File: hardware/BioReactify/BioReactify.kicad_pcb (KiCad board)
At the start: 4 copper layers, 110 x 110 mm, 131 parts, among them IC4 MJ5688-B111-HR1-C, J1 Conn_01x02, J10 Conn_01x06_Pin, J11 Conn_01x04_Pin, J12 Conn_01x04_Pin, J13 Conn_01x04_Pin, J14 Conn_01x04_Pin, J16 KF25C-7.62-2P, J17 Conn_01x02, J18 Conn_01x02, J19 Conn_01x02, J2 Conn_01x02, J20 Conn_01x02, J21 Conn_01x02, J22 Conn_01x02, J23 Conn_01x02, J24 Conn_01x03, J3 Conn_01x02, J4 Conn_01x02, J5 Conn_01x02, J6 Conn_01x03, J7 Conn_01x03, J8 Conn_01x02, J9 Conn_01x06_Pin, Q1 IRLZ44N, Q2 IRLZ44N, Q3 IRLZ44N, Q4 IRLZ44N, Q5 IRLZ44N, U1 LD1117S33TR_SOT223, U10 4N25, U11 4N25, U12 LD1117S50TR_SOT223, U13 MAX3490xSA, U14 TLV9001IDCK, U15 TLV9001IDCK, U16 TLV9001IDCK, U17 LD1117S33TR_SOT223, U18 MCP3208, U2 TLV9001IDCK, U3 TCA9544A, U4 TLV9001IDCK, U5 ESP32-DEVKIT-V1, U6 ACS712xLCBTR-030B3, U7 4N25, U8 4N25, U9 4N25

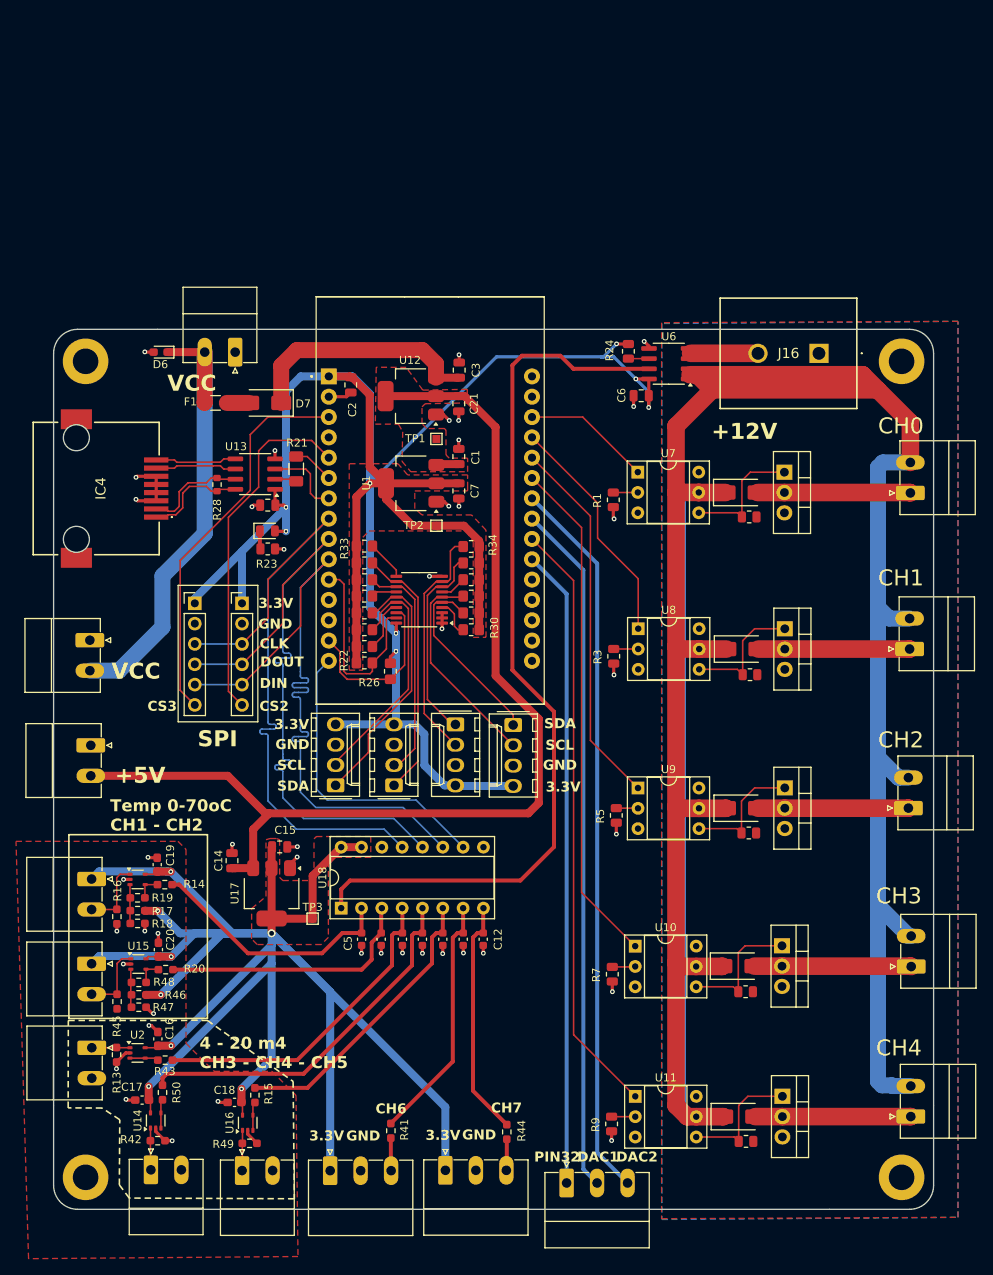
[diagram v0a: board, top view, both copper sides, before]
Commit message: Hardware updated
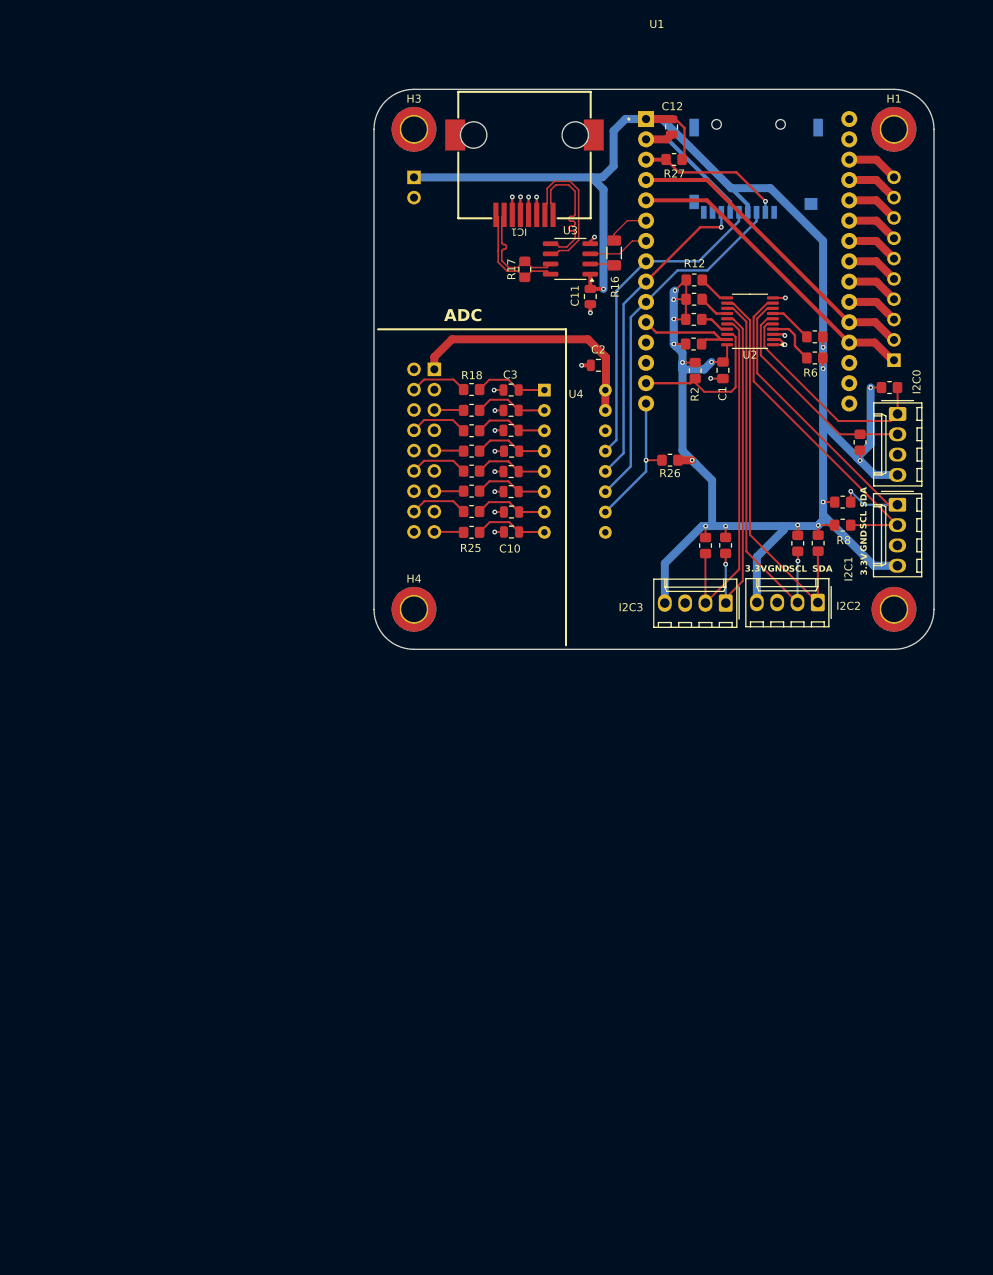
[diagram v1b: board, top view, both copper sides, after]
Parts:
- removed C13: 0.047uf, Capacitor_SMD:C_0603_1608Metric
- removed C14: 100nF, Capacitor_SMD:C_0805_2012Metric
- removed C15, C21: 10uF, Capacitor_SMD:C_0805_2012Metric
- removed C16, C17, C18, C19, C20: 0.1uF, Capacitor_SMD:C_0603_1608Metric_Pad1.08x0.95mm_HandSolder
- removed D1, D2, D3, D4, D5: 50V 5A, Diode_SMD:D_SMA
- removed D6: VS12VBA1HS, Diode_SMD:D_0603_1608Metric_Pad1.05x0.95mm_HandSolder
- removed D7: B340A-13-F, Diode_SMD:D_SMA
- removed D9: LED, LED_SMD:LED_0805_2012Metric
- removed F1: 13.2V 3A, Fuse:Fuse_1206_3216Metric
- removed IC4: MJ5688-B111-HR1-C, SamacSys_Parts:MJ5688B111HR1C
- removed J10, J9: Conn_01x06_Pin, Connector_PinHeader_2.54mm:PinHeader_1x06_P2.54mm_Vertical
- removed J11, J12, J13, J14: Conn_01x04_Pin, Connector_Molex:Molex_KK-254_AE-6410-04A_1x04_P2.54mm_Vertical
- removed J16: KF25C-7.62-2P, SamacSys_Parts:KF25C7622P
- removed J17, J18, J19, J20, J21, J22, J23, J5, J8: Conn_01x02, Connector_Phoenix_MC:PhoenixContact_MC_1,5_2-G-3.81_1x02_P3.81mm_Horizontal
- removed J24, J6, J7: Conn_01x03, Connector_Phoenix_MC:PhoenixContact_MC_1,5_3-G-3.81_1x03_P3.81mm_Horizontal
- removed Q1, Q2, Q3, Q4, Q5: IRLZ44N, Package_TO_SOT_THT:TO-220-3_Vertical
- removed R28: 120, Resistor_SMD:R_0603_1608Metric
- removed R29, R30, R31, R32, R33, R34, R35, R36, R37, R38, R39, R40: 10K, Resistor_SMD:R_0805_2012Metric_Pad1.20x1.40mm_HandSolder
- removed R41, R43, R44, R50: 1K, Resistor_SMD:R_0603_1608Metric_Pad0.98x0.95mm_HandSolder
- removed R42, R49: 150, Resistor_SMD:R_0603_1608Metric_Pad0.98x0.95mm_HandSolder
- removed R45: 7.8K, Resistor_SMD:R_0603_1608Metric_Pad0.98x0.95mm_HandSolder
- removed R46, R47: 4.1K, Resistor_SMD:R_0603_1608Metric_Pad0.98x0.95mm_HandSolder
- removed R48: 1.5K, Resistor_SMD:R_0603_1608Metric_Pad0.98x0.95mm_HandSolder
- removed TP1, TP2, TP3: TestPoint, TestPoint:TestPoint_Pad_1.0x1.0mm
- removed U10, U11, U7, U8, U9: 4N25, Package_DIP:DIP-6_W7.62mm_Socket
- removed U12: LD1117S50TR_SOT223, Package_TO_SOT_SMD:SOT-223-3_TabPin2
- removed U13: MAX3490xSA, Package_SO:SOIC-8_3.9x4.9mm_P1.27mm
- removed U14, U15, U16: TLV9001IDCK, Package_TO_SOT_SMD:SOT-353_SC-70-5
- removed U17: LD1117S33TR_SOT223, Package_TO_SOT_SMD:SOT-223-3_TabPin2
- removed U18: MCP3208, Package_DIP:DIP-16_W7.62mm_Socket
- removed U5: ESP32-DEVKIT-V1, other:MODULE_ESP32_DEVKIT_V1
- removed U6: ACS712xLCBTR-030B3, Package_SO:SOIC-8_3.9x4.9mm_P1.27mm
- added I2C0: Conn_01x04_Pin, Connector_Molex:Molex_KK-254_AE-6410-04A_1x04_P2.54mm_Vertical, F.Cu at (205.4, 60.6)
- added I2C1: Conn_01x04_Pin, Connector_Molex:Molex_KK-254_AE-6410-04A_1x04_P2.54mm_Vertical, F.Cu at (205.4, 71.9)
- added I2C2: Conn_01x04_Pin, Connector_Molex:Molex_KK-254_AE-6410-04A_1x04_P2.54mm_Vertical, F.Cu at (195.5, 84.2)
- added I2C3: Conn_01x04_Pin, Connector_Molex:Molex_KK-254_AE-6410-04A_1x04_P2.54mm_Vertical, F.Cu at (184.0, 84.2)
- added IC1: MJ5688-B111-HR1-C, custom:RJ45-TH_MJ5688-B111-HR1-C, F.Cu at (158.8, 30.7)
- added R11: 10K, Resistor_SMD:R_0805_2012Metric_Pad1.20x1.40mm_HandSolder, F.Cu at (193.0, 76.8)
- added R12: 10K, Resistor_SMD:R_0805_2012Metric_Pad1.20x1.40mm_HandSolder, F.Cu at (180.0, 43.8)
- added R25: 100, Resistor_SMD:R_0805_2012Metric_Pad1.20x1.40mm_HandSolder, F.Cu at (152.2, 75.4)
- C1: value 100nF -> 10uF; footprint Capacitor_SMD:C_0805_2012Metric -> Capacitor_SMD:C_0805_2012Metric_Pad1.18x1.45mm_HandSolder
- C10, C5, C8, C9: value 0.047uf -> 0.022uF; footprint Capacitor_SMD:C_0603_1608Metric -> Capacitor_SMD:C_0805_2012Metric
- C11, C12: value 0.047uf -> 10uF; footprint Capacitor_SMD:C_0603_1608Metric -> Capacitor_SMD:C_0805_2012Metric
- C3: value 100nF -> 0.022uF
- C4, C6, C7: value 10uF -> 0.022uF
- H1, H2, H3, H4: footprint MountingHole:MountingHole_3.2mm_M3_ISO7380_Pad -> MountingHole:MountingHole_3.2mm_M3_DIN965_Pad_TopBottom
- J1: value Conn_01x02 -> Conn_02x09_Odd_Even; footprint Connector_Phoenix_MC:PhoenixContact_MC_1,5_2-G-3.81_1x02_P3.81mm_Horizontal -> Connector_PinHeader_2.54mm:PinHeader_2x09_P2.54mm_Vertical; moved to B.Cu
- J2: value Conn_01x02 -> Conn_01x10_Pin; footprint Connector_Phoenix_MC:PhoenixContact_MC_1,5_2-G-3.81_1x02_P3.81mm_Horizontal -> Connector_PinHeader_2.54mm:PinHeader_1x10_P2.54mm_Vertical; moved to B.Cu
- J3: value Conn_01x02 -> Micro_SD_Card; footprint Connector_Phoenix_MC:PhoenixContact_MC_1,5_2-G-3.81_1x02_P3.81mm_Horizontal -> custom:TF-SMD_THD2528-11SD-GF; moved to B.Cu
- J4: value Conn_01x02 -> Conn_01x02_Pin; footprint Connector_Phoenix_MC:PhoenixContact_MC_1,5_2-G-3.81_1x02_P3.81mm_Horizontal -> Connector_PinHeader_2.54mm:PinHeader_1x02_P2.54mm_Vertical; moved to B.Cu
- R1, R3, R5, R7, R9: value 100 -> 10K; footprint Resistor_SMD:R_0805_2012Metric -> Resistor_SMD:R_0805_2012Metric_Pad1.20x1.40mm_HandSolder
- R10, R2, R4, R6, R8: value 470 -> 10K; footprint Resistor_SMD:R_0805_2012Metric -> Resistor_SMD:R_0805_2012Metric_Pad1.20x1.40mm_HandSolder
- R13: value 150 -> 10K; footprint Resistor_SMD:R_0603_1608Metric_Pad0.98x0.95mm_HandSolder -> Resistor_SMD:R_0805_2012Metric_Pad1.20x1.40mm_HandSolder
- R14, R15: value 1K -> 10K; footprint Resistor_SMD:R_0603_1608Metric_Pad0.98x0.95mm_HandSolder -> Resistor_SMD:R_0805_2012Metric_Pad1.20x1.40mm_HandSolder
- R16: value 7.8K -> 0; footprint Resistor_SMD:R_0603_1608Metric_Pad0.98x0.95mm_HandSolder -> Resistor_SMD:R_1206_3216Metric_Pad1.30x1.75mm_HandSolder
- R17, R18: value 4.1K -> 100; footprint Resistor_SMD:R_0603_1608Metric_Pad0.98x0.95mm_HandSolder -> Resistor_SMD:R_0805_2012Metric_Pad1.20x1.40mm_HandSolder
- R19: value 1.5K -> 100; footprint Resistor_SMD:R_0603_1608Metric_Pad0.98x0.95mm_HandSolder -> Resistor_SMD:R_0805_2012Metric_Pad1.20x1.40mm_HandSolder
- R20: value 1K -> 100; footprint Resistor_SMD:R_0603_1608Metric_Pad0.98x0.95mm_HandSolder -> Resistor_SMD:R_0805_2012Metric_Pad1.20x1.40mm_HandSolder
- R21: value 0 -> 100; footprint Resistor_SMD:R_1206_3216Metric_Pad1.30x1.75mm_HandSolder -> Resistor_SMD:R_0805_2012Metric_Pad1.20x1.40mm_HandSolder
- R22: value 10K -> 100
- R23: footprint Resistor_SMD:R_0805_2012Metric -> Resistor_SMD:R_0805_2012Metric_Pad1.20x1.40mm_HandSolder
- R24: value 10K -> 100; footprint Resistor_SMD:R_0805_2012Metric -> Resistor_SMD:R_0805_2012Metric_Pad1.20x1.40mm_HandSolder
- U1: value LD1117S33TR_SOT223 -> ESP32-DEVKIT-V1; footprint Package_TO_SOT_SMD:SOT-223-3_TabPin2 -> custom:MODULE_ESP32_DEVKIT_V1
- U2: value TLV9001IDCK -> TCA9544A; footprint Package_TO_SOT_SMD:SOT-353_SC-70-5 -> Package_SO:TSSOP-20_4.4x6.5mm_P0.65mm
- U3: value TCA9544A -> MAX3490xSA; footprint Package_SO:TSSOP-20_4.4x6.5mm_P0.65mm -> Package_SO:SOIC-8_3.9x4.9mm_P1.27mm
- U4: value TLV9001IDCK -> MCP3208; footprint Package_TO_SOT_SMD:SOT-353_SC-70-5 -> Package_DIP:DIP-16_W7.62mm_Socket
- moved H1 165.4 mm to (205.0, 25.0)
- moved J3 140.6 mm to (187.8, 30.1)
- moved J2 137.4 mm to (205.0, 53.9)
- moved U2 119.3 mm to (187.0, 49.0), turned to 180 degrees
- moved R15 113.6 mm to (180.0, 46.2), turned to 0 degrees
- moved H2 105.7 mm to (205.0, 85.0)
- moved C12 104.2 mm to (177.2, 24.7)
- moved R16 103.7 mm to (170.0, 40.5), turned to -90 degrees
- moved R9 101.6 mm to (195.1, 50.9), turned to 180 degrees
- moved R13 99.2 mm to (183.9, 77.0), turned to -90 degrees
- moved J4 96.5 mm to (145.0, 31.0), turned to 180 degrees
- moved J1 95.0 mm to (147.5, 55.0), turned to 180 degrees
- moved R17 93.6 mm to (158.8, 42.5), turned to 90 degrees
- moved H4 93.6 mm to (145.0, 85.0)
- moved C11 83.7 mm to (167.0, 45.9)
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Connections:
- C1 pad 1: +5V -> VDD
- C10 pad 1: /adc0/CH6 -> /ADC/CH7
- C11 pad 1: /adc0/CH3 -> VDD
- C12 pad 1: /adc0/CH7 -> VDD
- C2 pad 1: +3.3V -> +3.3VADC
- C3 pad 1: /Vcc_protected -> /ADC/CH0
- C4 pad 1: +3.3V -> /ADC/CH1
- C5 pad 1: /adc0/CH1 -> /ADC/CH2
- C6 pad 1: +3.3V -> /ADC/CH3
- C7 pad 1: +3.3V -> /ADC/CH4
- C8 pad 1: /adc0/CH5 -> /ADC/CH5
- C9 pad 1: /adc0/CH2 -> /ADC/CH6
- H1 pad 1: unconnected-(H1-Pad1) -> GND
- H2 pad 1: unconnected-(H2-Pad1) -> GND
- H3 pad 1: unconnected-(H3-Pad1) -> GND
- H4 pad 1: unconnected-(H4-Pad1) -> GND
- J1 pad 1: /adc0/IN1 -> +3.3VADC
- J2 pad 1: /adc0/IN2 -> /D4
- J2 pad 2: GND -> /D2
- J3 pad 1: /adc0/IN3 -> unconnected-(J3-DAT2-Pad1)
- J3 pad 2: GND -> /CS1
- J4 pad 1: +3.3VADC -> VDD
- J4 pad 2: /adc0/IN4 -> GND
- R1 pad 1: /SQ0 -> VDD
- R1 pad 2: GND -> /SDA
- R10 pad 1: /PQ4 -> VDD
- R10 pad 2: GNDPWR -> /I2C/SD2
- R13 pad 1: GND -> VDD
- R13 pad 2: /adc0/IN1 -> /I2C/SD3
- R14 pad 1: /adc0/CH1 -> VDD
- R14 pad 2: /adc0/TCH1 -> /I2C/SC3
- R15 pad 1: /adc0/CH5 -> VDD
- R15 pad 2: /adc0/ICH5 -> /I2C/INT3
- R16 pad 1: GND -> /RS485/RX2
- R16 pad 2: /adc0/IN4 -> /RS485/R0
- R17 pad 1: Net-(U4--) -> /RS485/RX_P
- R17 pad 2: +3.3VADC -> /RS485/RX_N
- R18 pad 1: GND -> /ADC/CH0
- R18 pad 2: Net-(U4--) -> /ADC/INCH0
- R19 pad 1: Net-(U4--) -> /ADC/CH1
- R19 pad 2: /adc0/TCH1 -> /ADC/INCH1
- R2 pad 1: /PQ0 -> VDD
- R2 pad 2: GNDPWR -> /SCL
- R20 pad 1: /adc0/CH2 -> /ADC/CH2
- R20 pad 2: /adc0/TCH2 -> /ADC/INCH2
- R21 pad 1: /RX2 -> /ADC/CH3
- R21 pad 2: /R0 -> /ADC/INCH3
- R22 pad 1: +3.3V -> /ADC/CH4
- R22 pad 2: /SDA -> /ADC/INCH4
- R23 pad 1: GND -> /ADC/CH5
- R23 pad 2: /led_3v3 -> /ADC/INCH5
- R24 pad 1: +3.3V -> /ADC/CH6
- R24 pad 2: Net-(U6-FAULT) -> /ADC/INCH6
- R26 pad 1: +3.3V -> VDD
- R26 pad 2: /SCL -> /CS
- R27 pad 1: +3.3V -> VDD
- R27 pad 2: /i2c/SC0 -> /CS1
- R3 pad 1: /SQ1 -> VDD
- R3 pad 2: GND -> Net-(U2-~{INT})
- R4 pad 1: /PQ1 -> VDD
- R4 pad 2: GNDPWR -> /I2C/SD0
- R5 pad 1: /SQ2 -> VDD
- R5 pad 2: GND -> /I2C/SC0
- R6 pad 1: /PQ2 -> VDD
- R6 pad 2: GNDPWR -> /I2C/INT0
- R7 pad 1: /SQ3 -> VDD
- R7 pad 2: GND -> /I2C/SD1
- R8 pad 1: /PQ3 -> VDD
- R8 pad 2: GNDPWR -> /I2C/SC1
- R9 pad 1: /SQ4 -> VDD
- R9 pad 2: GND -> /I2C/INT1
- U1 pad 1: GND -> VDD
- U1 pad 2: +3.3V -> GND
- U1 pad 3: +5V -> /CS1
- U2 pad 1: /adc0/IN1 -> GND
- U2 pad 3: /adc0/ICH3 -> GND
- U2 pad 4: /adc0/ICH3 -> /I2C/INT0
- U2 pad 5: +3.3VADC -> /I2C/SD0
- U3 pad 1: GND -> VDD
- U3 pad 2: GND -> /RS485/R0
- U3 pad 3: GND -> /RS485/TX2
- U3 pad 4: /i2c/INT0 -> GND
- U3 pad 5: /i2c/SD0 -> /RS485/TX_P
- U3 pad 6: /i2c/SC0 -> /RS485/TX_N
- U3 pad 7: /i2c/INT1 -> /RS485/RX_N
- U3 pad 8: /i2c/SD1 -> /RS485/RX_P
- U4 pad 1: /adc0/IN4 -> /ADC/CH0
- U4 pad 2: GND -> /ADC/CH1
- U4 pad 3: Net-(U4--) -> /ADC/CH2
- U4 pad 4: /adc0/TCH1 -> /ADC/CH3
- U4 pad 5: +3.3VADC -> /ADC/CH4
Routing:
- net +12V: track 371.7 -> 0.00 mm
- net VDD: track 0.00 -> 273.1 mm, vias 0 -> 17
- net +3.3V: track 264.9 -> 0.00 mm, vias 8 -> 0
- net +3.3VADC: track 254.2 -> 31.5 mm, vias 8 -> 0
- net +5V: track 136.4 -> 0.00 mm
- net /CH0: track 111.7 -> 0.00 mm
- net /SPI_DIN: track 87.5 -> 0.00 mm
- net /SPI_DOUT: track 87.5 -> 0.00 mm
- net /SPI_CLK: track 87.0 -> 0.00 mm
- net /DAC2: track 90.5 -> 6.51 mm
- net /DAC1: track 86.4 -> 6.51 mm
- net /PIN32: track 79.8 -> 0.00 mm
- net /Q4: track 75.0 -> 0.00 mm
- net /Q3: track 63.9 -> 0.00 mm
- net VCC: track 58.9 -> 0.00 mm
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- removed copper zone on B.Cu, net +12V
- removed copper zone on F.Cu, net +3.3V
- removed copper zone on F.Cu, net +3.3VADC
- removed copper zone on F.Cu, net +5V
- removed copper zone on F.Cu, net GND
- removed copper zone on F.Cu, net GNDPWR
- removed copper zone on In1.Cu, net GNDPWR
- removed copper zone on In2.Cu, net GNDPWR
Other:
- board size 110 x 110 mm -> 70 x 70 mm
- board text added: "ADC"
- board text removed: "+12V"
- board text removed: "+5V"
- board text removed: "4 - 20 m4 CH3 - CH4 - CH5"
- board text removed: "CH0"
- board text removed: "CH1"
- board text removed: "CH2"
- board text removed: "CH3"
- board text removed: "CH4"
- board text removed: "CH6"
- board text removed: "CH7"
- board text removed: "CLK"
- board text removed: "CS2"
- board text removed: "CS3"
- board text removed: "DAC1"
- board text removed: "DAC2"
- board text removed: "DIN"
- board text removed: "DOUT"
- board text removed: "PIN32"
- board text removed: "SPI"
- board text removed: "Temp 0-70oC CH1 - CH2"
- board text removed: "VCC"
